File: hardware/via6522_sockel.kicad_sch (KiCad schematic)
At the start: 6 parts, among them IC1 VIA6522, P1 VIA_PIN_1-20, P2 VIA_PIN_21-40, Q1 BSS138, U2 SN74LVC4245A

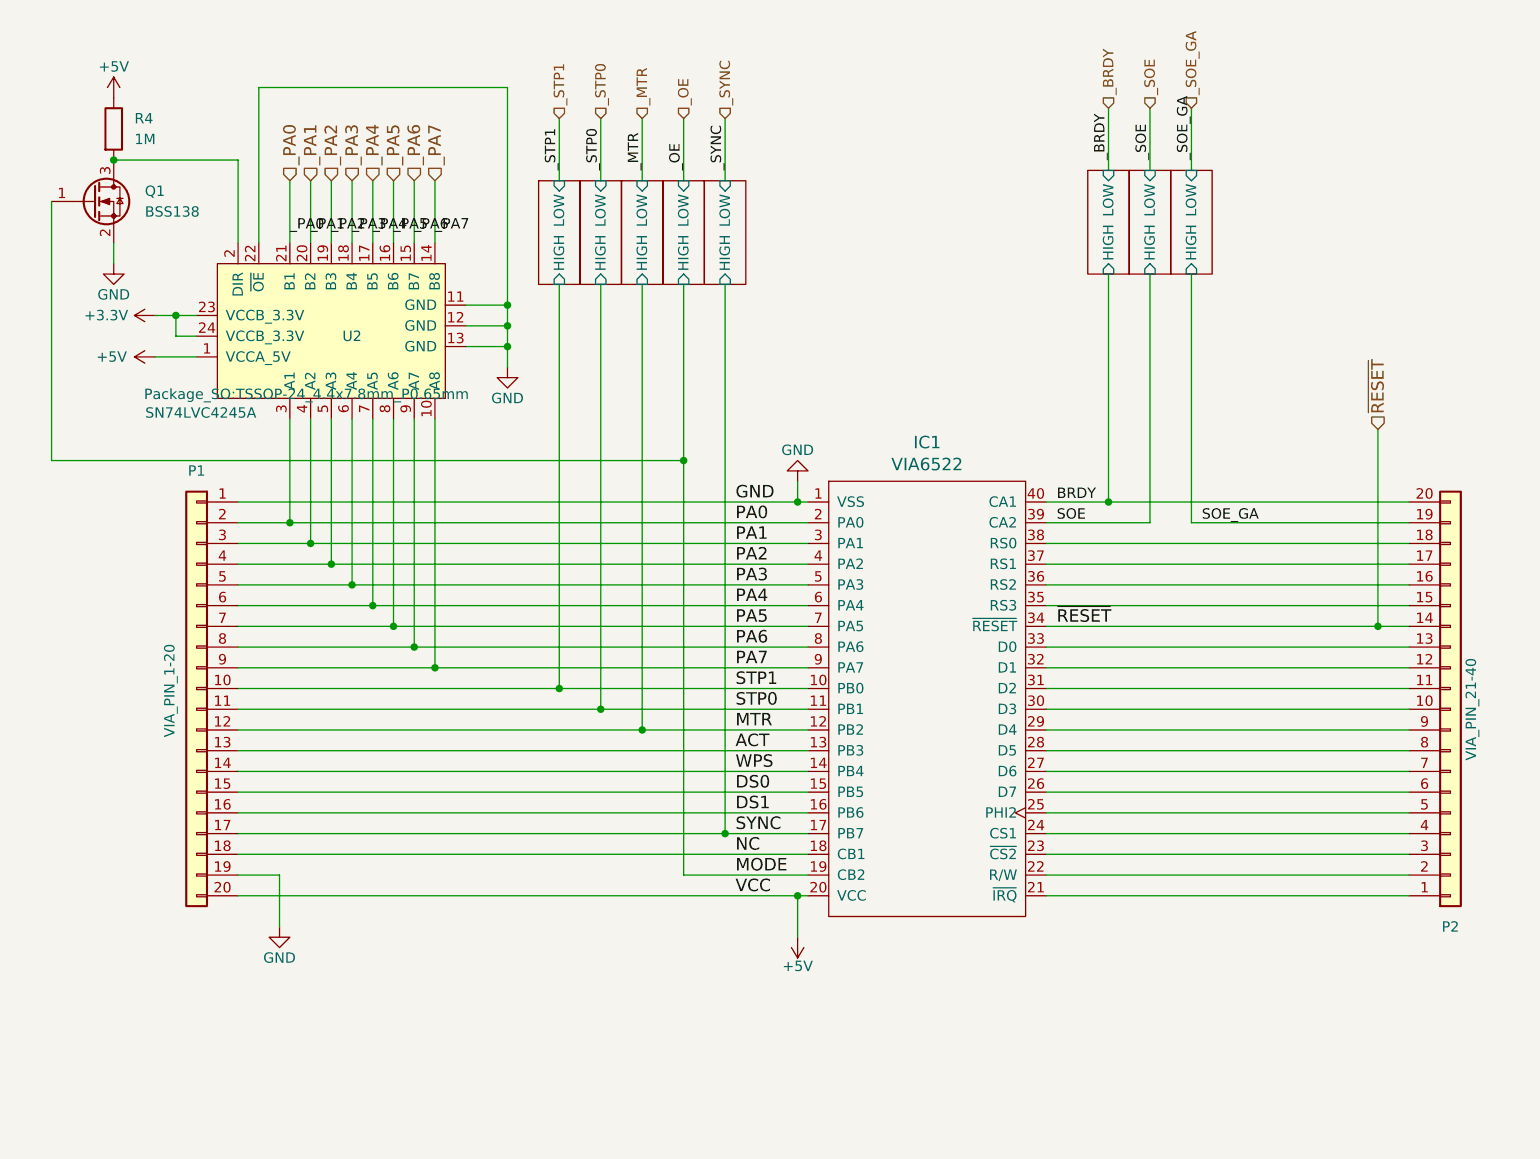
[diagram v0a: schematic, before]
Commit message: updated PDFs for PCB v1.6
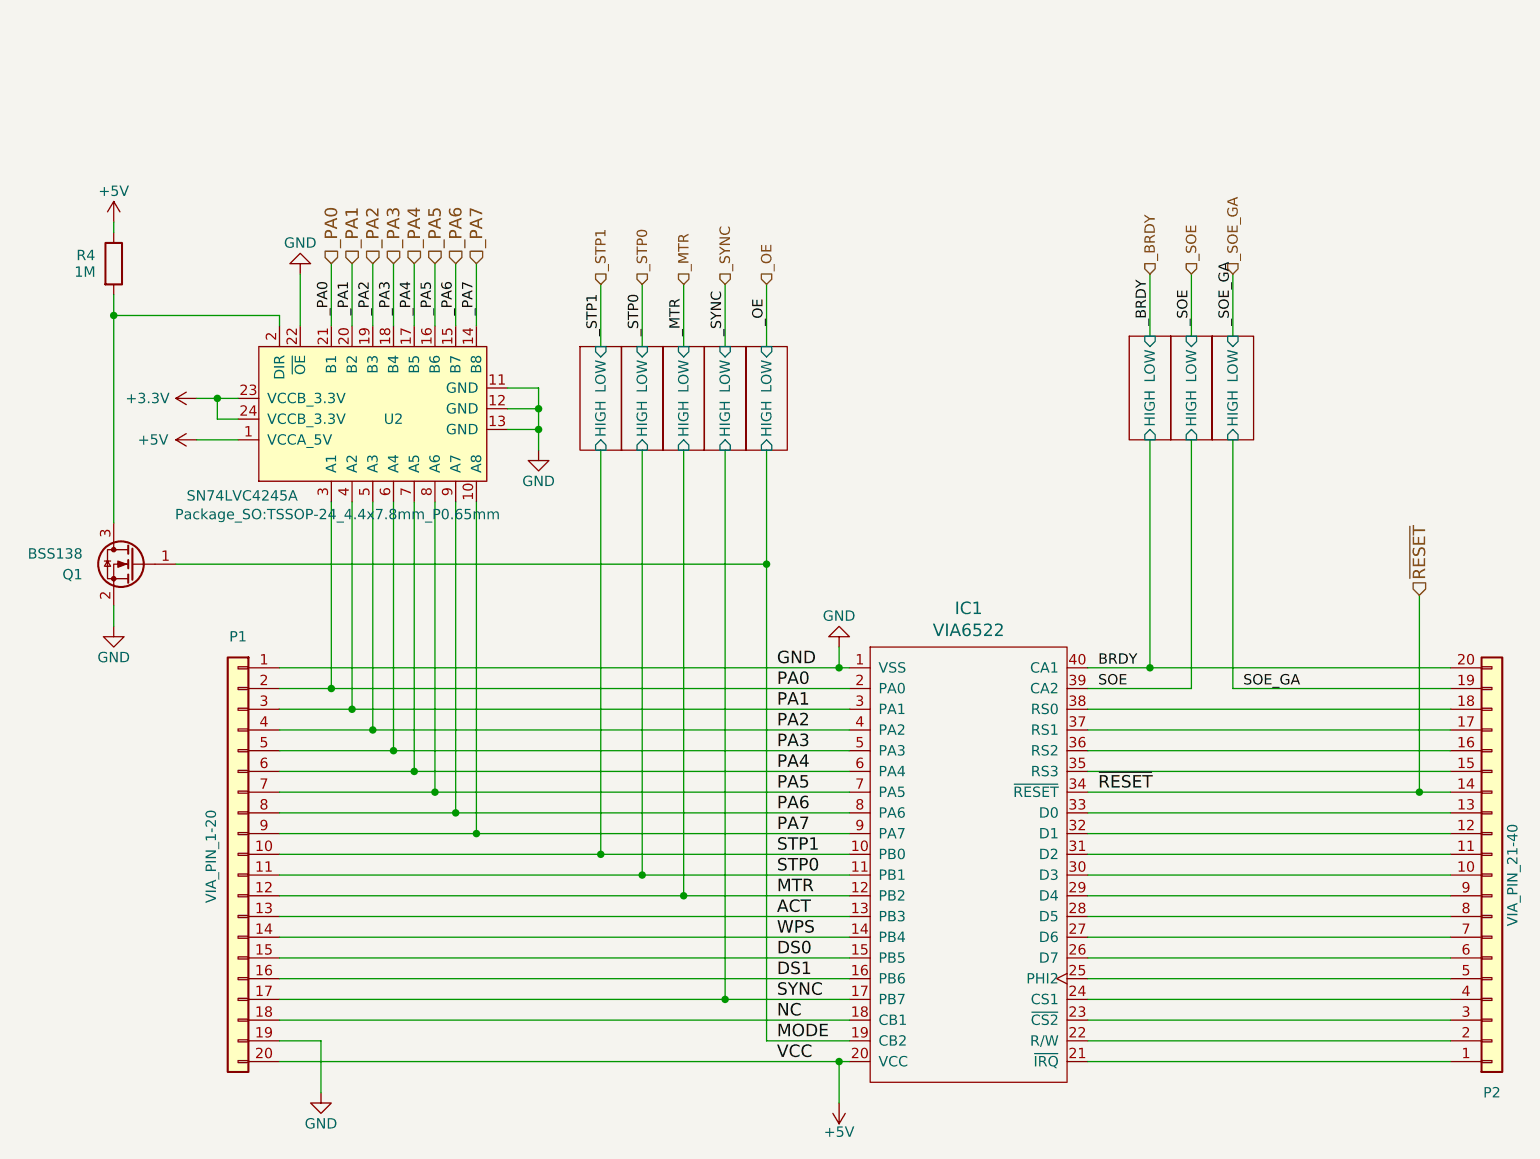
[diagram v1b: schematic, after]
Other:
- moved on the sheet: IC1, P1, P2, Q1, R4, U2
